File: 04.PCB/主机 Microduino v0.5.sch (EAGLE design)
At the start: 22 parts

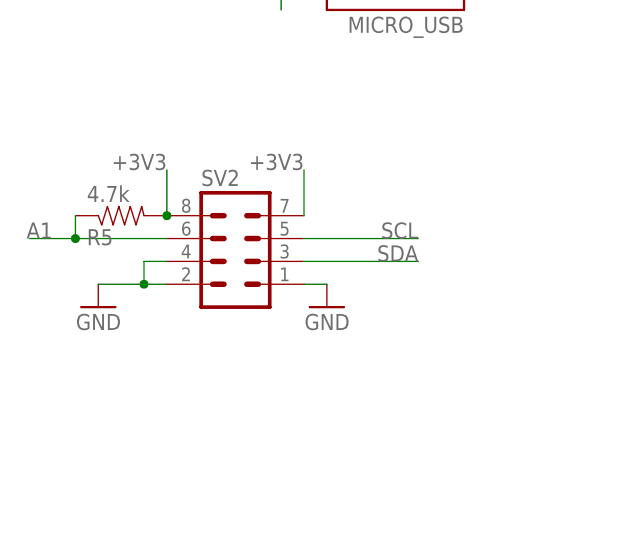
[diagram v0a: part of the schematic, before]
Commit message: 更新
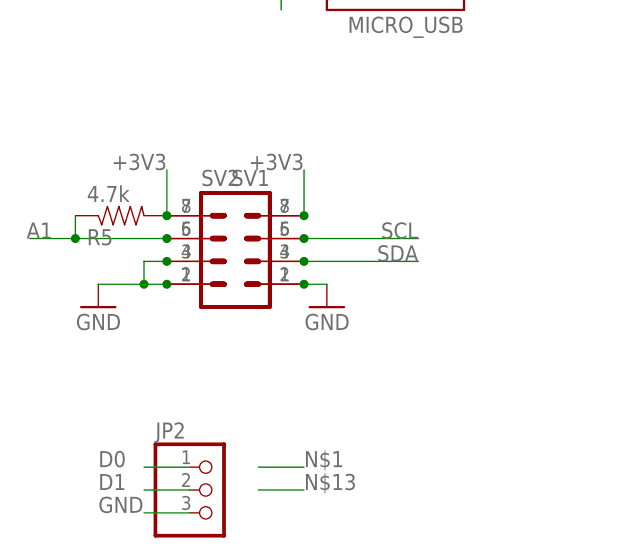
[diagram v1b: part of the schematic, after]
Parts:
- added JP2: (no value), pinhead:PINHD-1X3
- added SV1: (no value), pkj:MA04-2
- C1, C2: device microduino:CAP_POL1206 -> microduino:CAP_POL3528
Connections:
- net +3V3: now also SV1.7, SV1.8
- net A1: now also SV1.5
- net D0: now also JP2.1
- net D1: now also JP2.2
- net GND: now also JP2.3, SV1.1, SV1.2, SV1.3
- net SCL: now also SV1.6
- net SDA: now also SV1.4
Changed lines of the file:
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@@
 <part name="DC-3V3" library="00my" deviceset="REG1117" device="SOT223"/>
 <part name="USB" library="microduino" deviceset="MICRO_USB" device=""/>
-<part name="C1" library="microduino" deviceset="CAP_POL" device="1206"/>
-<part name="C2" library="microduino" deviceset="CAP_POL" device="1206"/>
+<part name="C1" library="microduino" deviceset="CAP_POL" device="3528"/>
+<part name="C2" library="microduino" deviceset="CAP_POL" device="3528"/>
 <part name="C3" library="microduino" deviceset="CAP" device="0603-CAP"/>
 <part name="C4" library="microduino" deviceset="CAP" device="0603-CAP"/>
@@
 <part name="C7" library="microduino" deviceset="CAP" device="0603-CAP"/>
 <part name="GND8" library="microduino" deviceset="GND" device=""/>
+<part name="SV1" library="pkj" deviceset="MA04-2" device="">
+<attribute name="MF" value=""/>
+<attribute name="MPN" value=""/>
+<attribute name="OC_FARNELL" value="unknown"/>
+<attribute name="OC_NEWARK" value="unknown"/>
+</part>
+<part name="JP2" library="pinhead" deviceset="PINHD-1X3" device=""/>
 </parts>
 <sheets>
@@
 <instance part="C7" gate="G$1" x="71.12" y="5.08"/>
 <instance part="GND8" gate="1" x="71.12" y="0"/>
+<instance part="SV1" gate="G$1" x="-5.08" y="7.62" rot="MR0"/>
+<instance part="JP2" gate="A" x="-7.62" y="-20.32"/>
 </instances>
 <busses>
@@
 <pinref part="SV2" gate="G$1" pin="2"/>
 <pinref part="SV2" gate="G$1" pin="4"/>
+<pinref part="SV1" gate="G$1" pin="1"/>
+<junction x="-12.7" y="2.54"/>
+<pinref part="SV1" gate="G$1" pin="3"/>
+<junction x="-12.7" y="5.08"/>
 </segment>
 <segment>
@@
 <pinref part="GND19" gate="1" pin="GND"/>
 <pinref part="SV2" gate="G$1" pin="1"/>
+<pinref part="SV1" gate="G$1" pin="2"/>
+<junction x="2.54" y="2.54"/>
 </segment>
 <segment>
@@
 <pinref part="C7" gate="G$1" pin="2"/>
 <pinref part="GND8" gate="1" pin="GND"/>
+</segment>
+<segment>
+<pinref part="JP2" gate="A" pin="3"/>
+<wire x1="-10.16" y1="-22.86" x2="-15.24" y2="-22.86" width="0.1524" layer="91"/>
+<label x="-20.32" y="-22.86" size="1.778" layer="95"/>
 </segment>
 </net>
@@
 <junction x="-22.86" y="7.62"/>
 <pinref part="SV2" gate="G$1" pin="6"/>
+<pinref part="SV1" gate="G$1" pin="5"/>
+<junction x="-12.7" y="7.62"/>
 </segment>
 </net>
@@
 <label x="142.24" y="121.92" size="1.778" layer="95"/>
 </segment>
+<segment>
+<wire x1="-10.16" y1="-17.78" x2="-15.24" y2="-17.78" width="0.1524" layer="91"/>
+<label x="-20.32" y="-17.78" size="1.778" layer="95"/>
+<pinref part="JP2" gate="A" pin="1"/>
+</segment>
 </net>
 <net name="D1" class="0">
@@
 <wire x1="147.32" y1="127" x2="149.86" y2="129.54" width="0.1524" layer="91"/>
 <label x="142.24" y="127" size="1.778" layer="95"/>
+</segment>
+<segment>
+<wire x1="-10.16" y1="-20.32" x2="-15.24" y2="-20.32" width="0.1524" layer="91"/>
+<label x="-20.32" y="-20.32" size="1.778" layer="95"/>
+<pinref part="JP2" gate="A" pin="2"/>
 </segment>
 </net>
@@
 <wire x1="2.54" y1="10.16" x2="2.54" y2="15.24" width="0.1524" layer="91"/>
 <pinref part="SV2" gate="G$1" pin="7"/>
+<pinref part="SV1" gate="G$1" pin="8"/>
+<junction x="2.54" y="10.16"/>
 </segment>
 <segment>
@@
 <pinref part="SV2" gate="G$1" pin="8"/>
 <junction x="-12.7" y="10.16"/>
+<pinref part="SV1" gate="G$1" pin="7"/>
 </segment>
 <segment>
@@
 <label x="15.24" y="7.62" size="1.778" layer="95" rot="MR0"/>
 <pinref part="SV2" gate="G$1" pin="5"/>
+<pinref part="SV1" gate="G$1" pin="6"/>
+<junction x="2.54" y="7.62"/>
 </segment>
 </net>
@@
 <label x="15.24" y="5.08" size="1.778" layer="95" rot="MR0"/>
 <pinref part="SV2" gate="G$1" pin="3"/>
-</segment>
-</net>
+<pinref part="SV1" gate="G$1" pin="4"/>
+<junction x="2.54" y="5.08"/>
+</segment>
+</net>
+<net name="N$1" class="0">
+<segment>
+<wire x1="-2.54" y1="-17.78" x2="2.54" y2="-17.78" width="0.1524" layer="91"/>
+<label x="2.54" y="-17.78" size="1.778" layer="95"/>
+</segment>
+</net>
+<net name="N$13" class="0">
+<segment>
+<wire x1="-2.54" y1="-20.32" x2="2.54" y2="-20.32" width="0.1524" layer="91"/>
+<label x="2.54" y="-20.32" size="1.778" layer="95"/>
+</segment>
+</net>
